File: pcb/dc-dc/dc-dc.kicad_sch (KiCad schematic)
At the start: 51 parts, among them J8 power, U4 LMR16030SDDAR, U5 LMR16030SDDAR, U6 LMR16030SDDAR

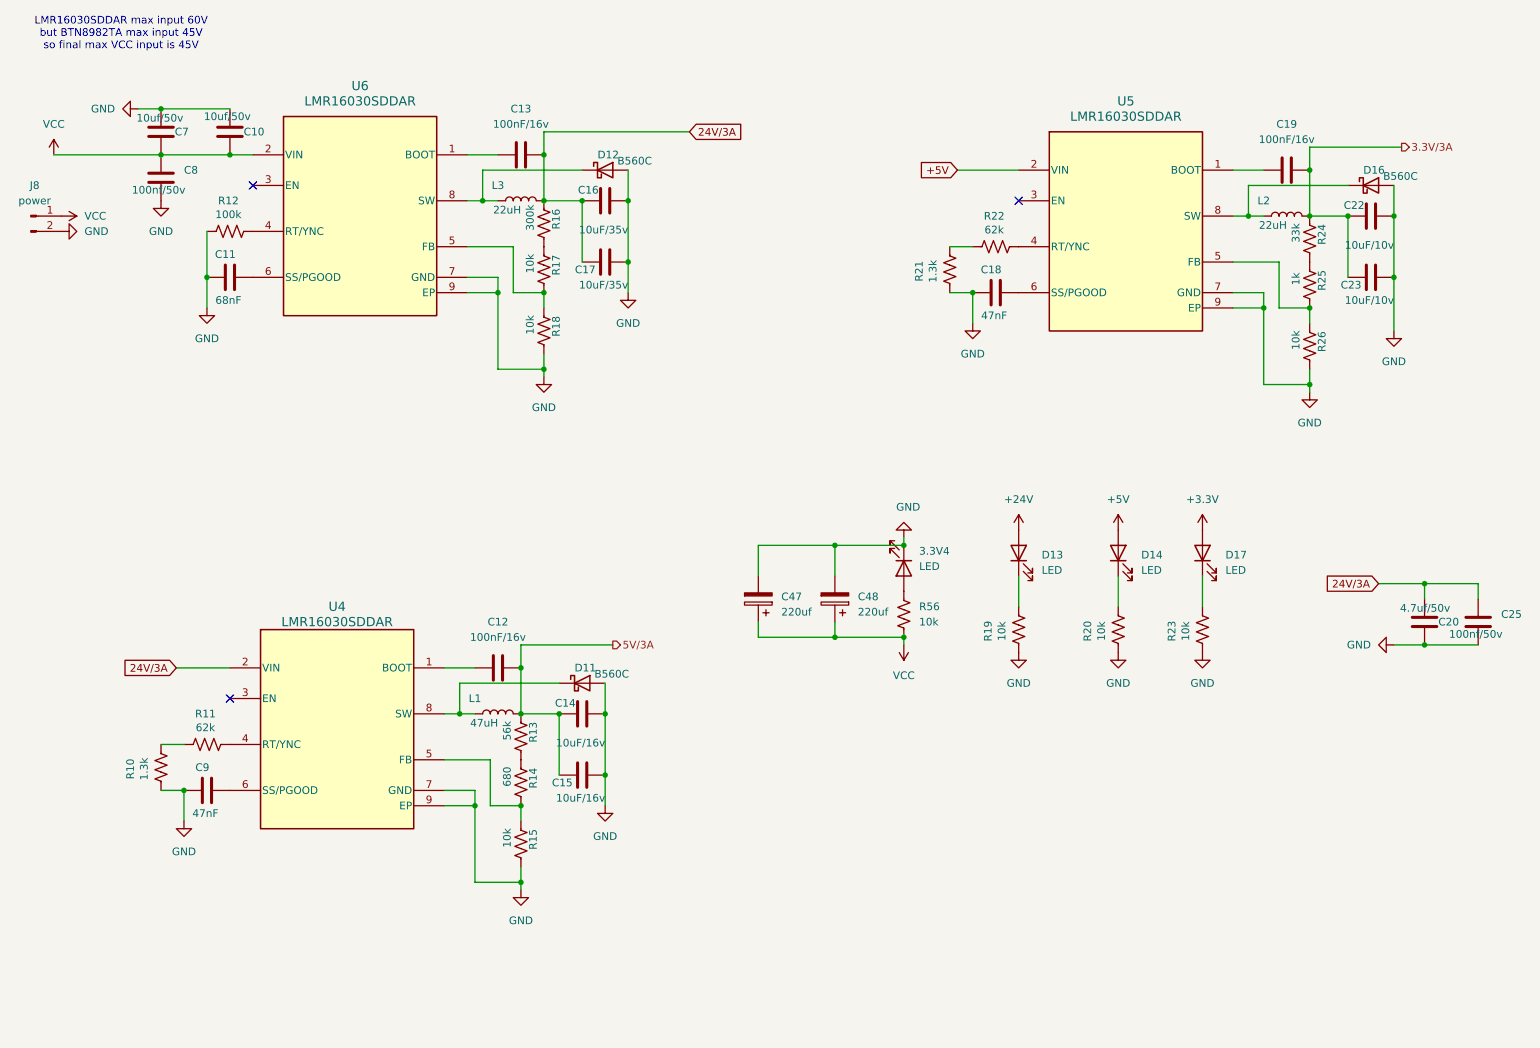
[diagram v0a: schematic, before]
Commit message: feat: update
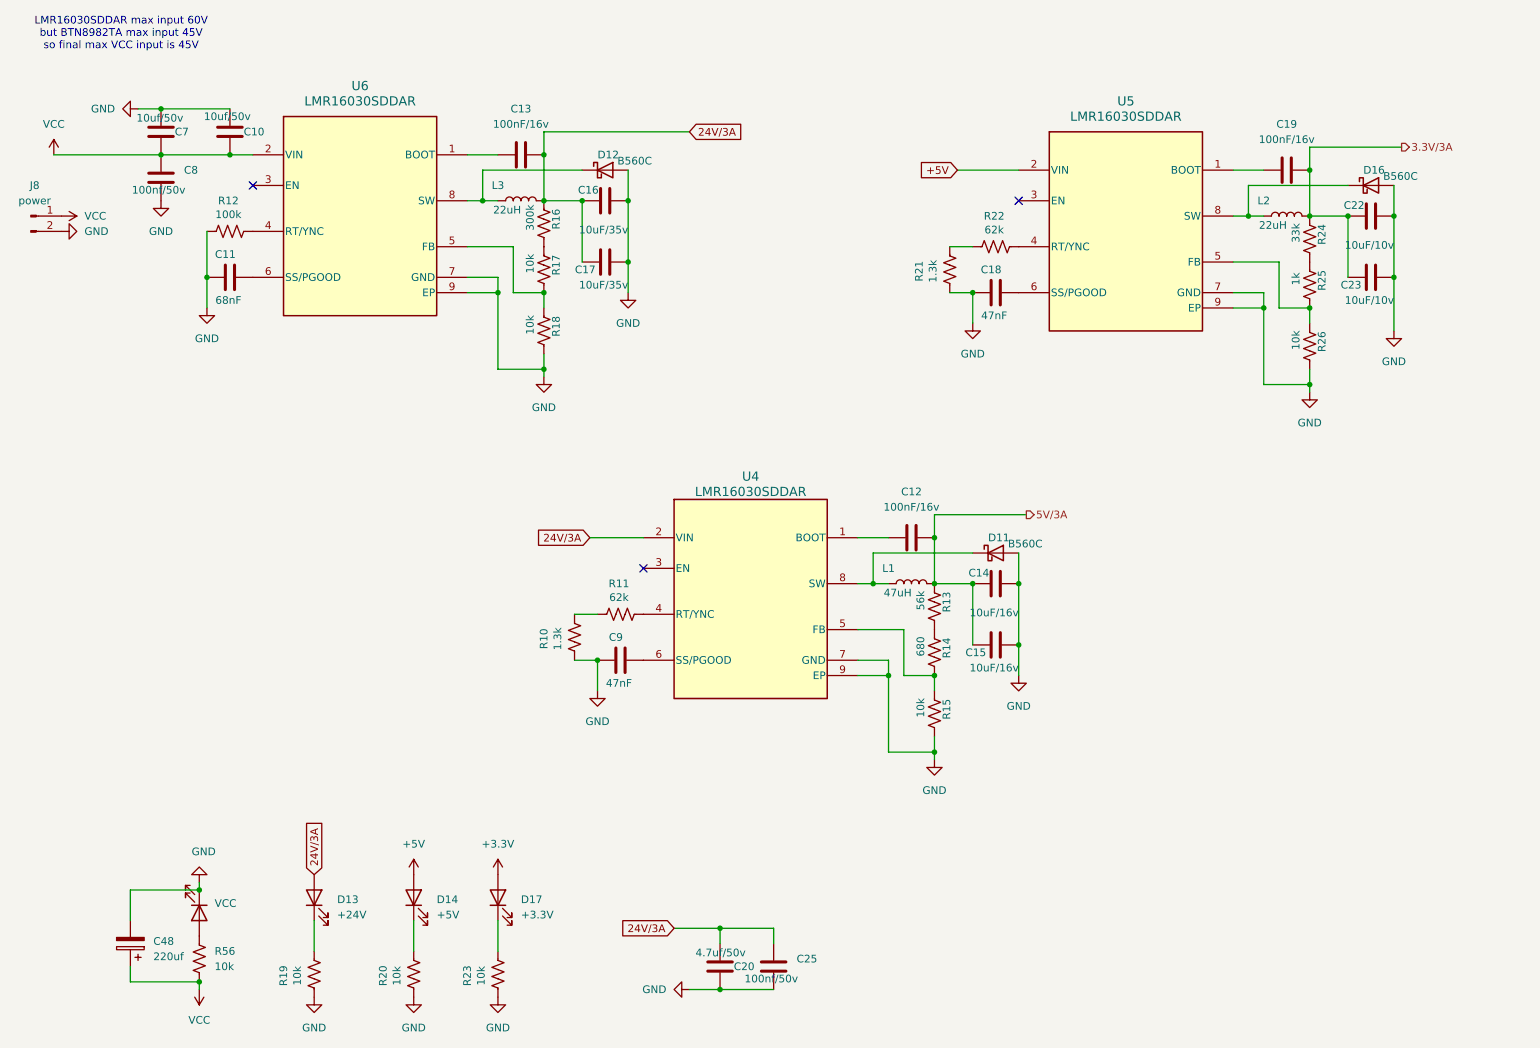
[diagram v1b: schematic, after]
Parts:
- removed C47: 220uf, Capacitor_SMD:CP_Elec_10x10.5, symbol Device:C_Polarized
- 3.3V4: value LED -> VCC
- D13: value LED -> +24V
- D14: value LED -> +5V
- D17: value LED -> +3.3V
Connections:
- net +24V is gone; now on net 24V/3A: D13.2 (A)
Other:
- moved on the sheet: C12, C14, C15, C20, C25, C48, C9, D11, D13, D14, D17, L1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
